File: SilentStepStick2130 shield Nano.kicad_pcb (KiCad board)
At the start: 4 copper layers, 34.5 x 49.4 mm, 11 parts, among them J1 Conn_01x04_Socket, J2 Conn_01x04_Socket, J3 Conn_01x02_Pin, J4 Conn_01x02_Pin, J5 Conn_01x03, J6 Conn_01x02_Pin, U1 TMC2130_SILENTSTEPSTICK, U2 TMC2130_SILENTSTEPSTICK

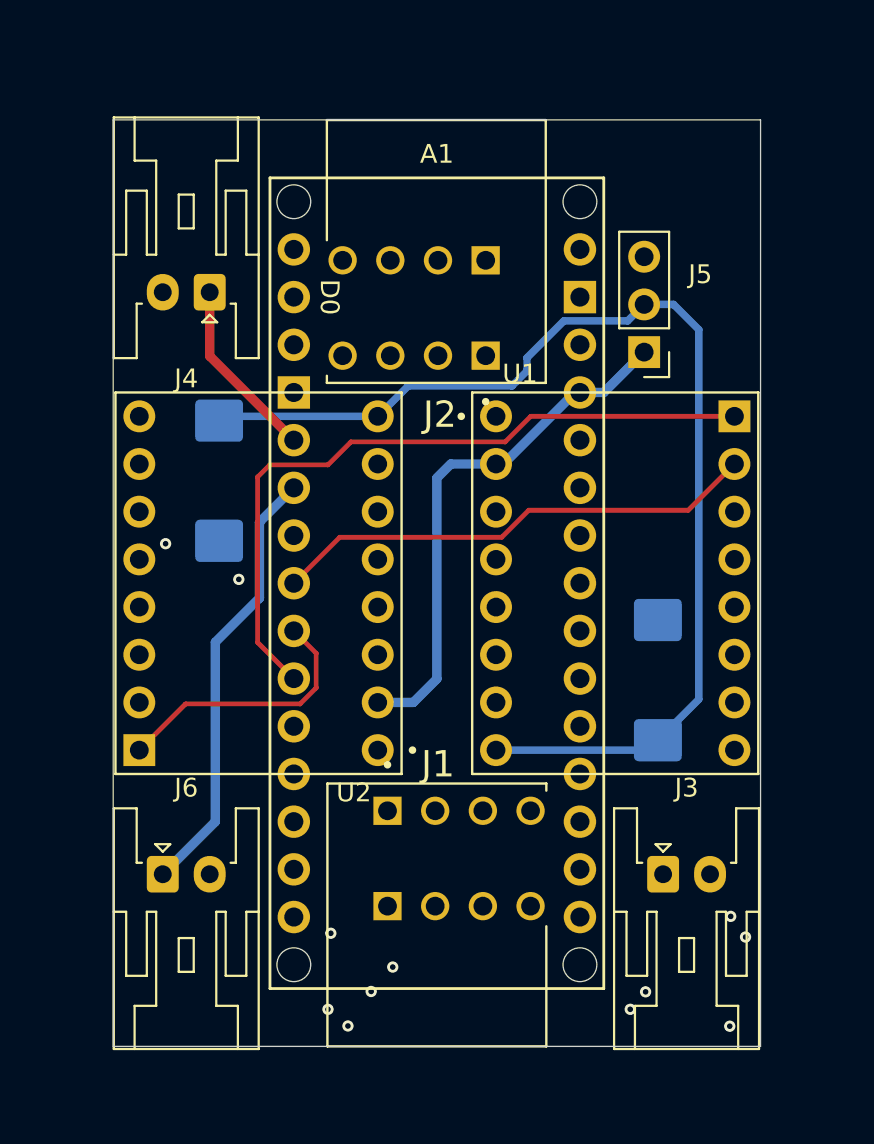
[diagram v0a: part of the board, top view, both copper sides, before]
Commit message: v1
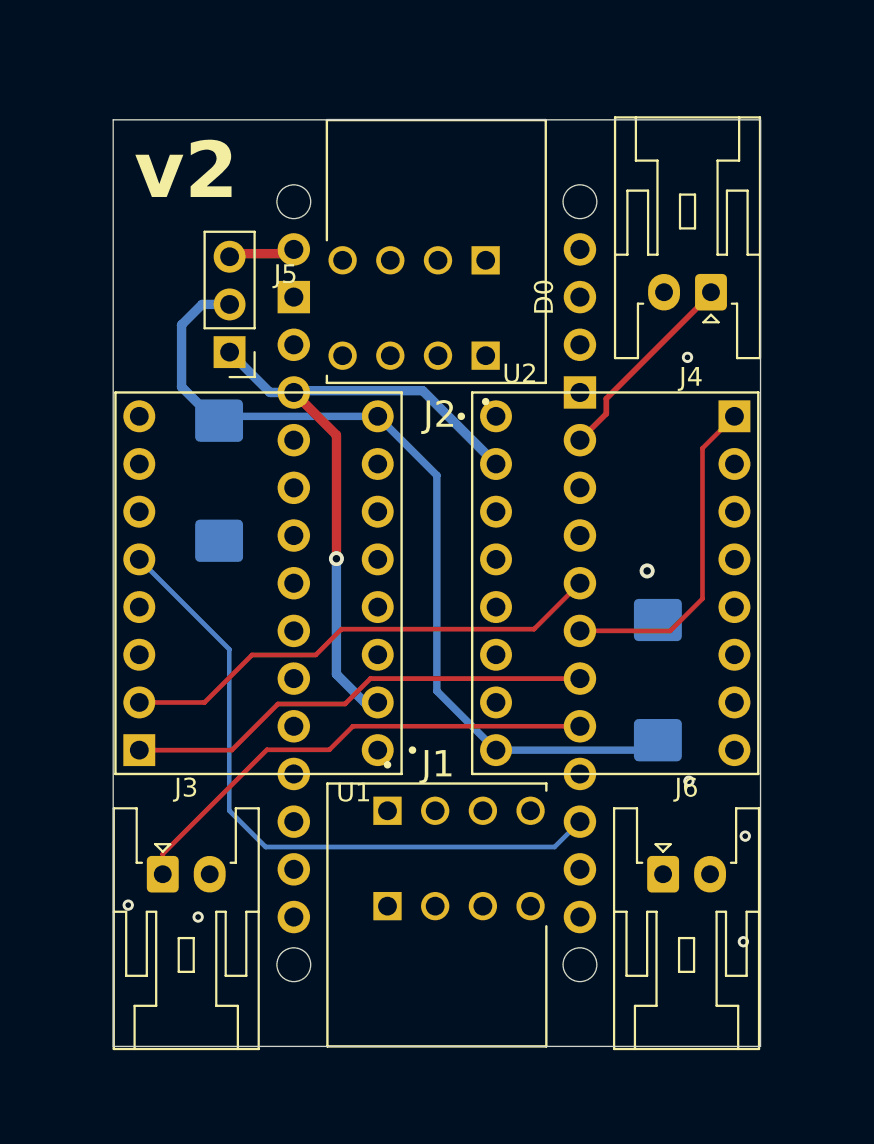
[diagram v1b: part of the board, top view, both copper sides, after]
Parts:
- added REF**: KiCad-Logo2_5mm_SilkScreen, Symbol:KiCad-Logo2_5mm_SilkScreen, B.Cu at (161.9, 93.6)
- A1: moved to B.Cu
- moved J4 26.7 mm to (164.6, 84.5)
- moved J3 26.7 mm to (135.4, 115.5)
- moved J6 26.7 mm to (162.1, 115.5)
- moved J5 22.1 mm to (139.0, 87.7)
- moved U1 19.0 mm to (140.5, 100.0), turned to 180 degrees
- moved U2 19.0 mm to (159.5, 100.0), turned to 0 degrees
- turned A1 to 180 degrees
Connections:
- J1 pad 1: /OA2_1 -> /OB2_1
- J1 pad 2: /OA1_1 -> /OB1_1
- J1 pad 3: /OB1_1 -> /OA1_1
- J1 pad 4: /OB2_1 -> /OA2_1
- J2 pad 1: /OA2_2 -> /OB2_2
- J2 pad 2: /OA1_2 -> /OB1_2
- J2 pad 3: /OB1_2 -> /OA1_2
- J2 pad 4: /OB2_2 -> /OA2_2
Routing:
- net /MOSI: track 66.8 -> 91.2 mm
- net /CS_1: track 58.1 -> 35.4 mm, vias 2 -> 0
- net /VM: track 60.7 -> 46.8 mm
- net /DIR_1: track 38.3 -> 25.0 mm
- net Net-(J3-Pin_1): track 37.9 -> 26.1 mm, vias 2 -> 0
- net /OA2_2: track 15.8 -> 25.2 mm
- net /OA2_1: track 15.8 -> 25.2 mm
- net +5V: track 28.2 -> 35.5 mm, vias 0 -> 1
- net /OB2_2: track 21.8 -> 15.2 mm
- net /MISO: track 75.0 -> 68.9 mm, vias 2 -> 1
- net /OB2_1: track 21.8 -> 15.8 mm
- net /STEP_2: track 16.0 -> 10.7 mm, vias 1 -> 0
- net /OB1_2: track 21.0 -> 17.2 mm
- net /OB1_1: track 21.0 -> 17.2 mm
- net /OA1_2: track 17.3 -> 20.8 mm
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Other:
- board text added: "v2"
